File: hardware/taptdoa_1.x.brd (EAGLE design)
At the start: 64.8 x 63.2 mm, 60 parts, among them J1 105017-0001, U1 AP2112K-3.3TRG1, U2 STM32F103RBT6, Y1 8MHz

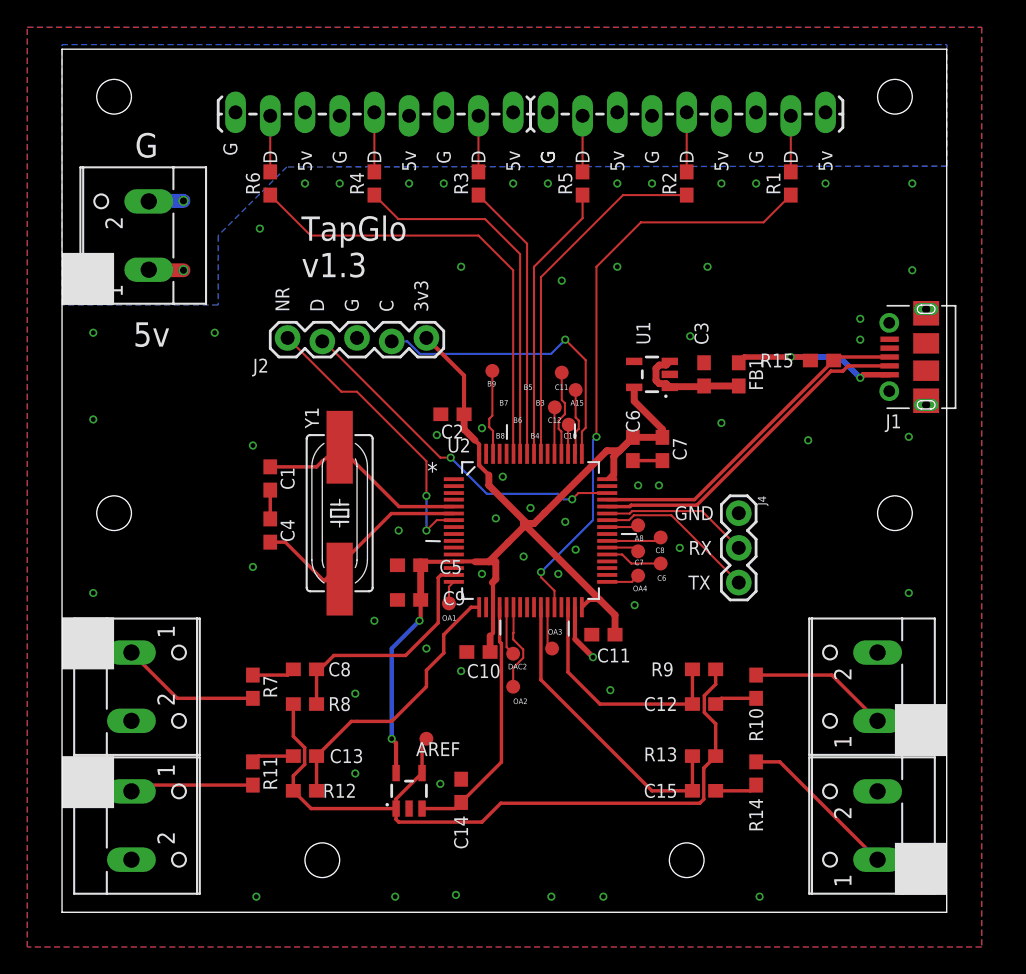
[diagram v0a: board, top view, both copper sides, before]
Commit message: re layout board
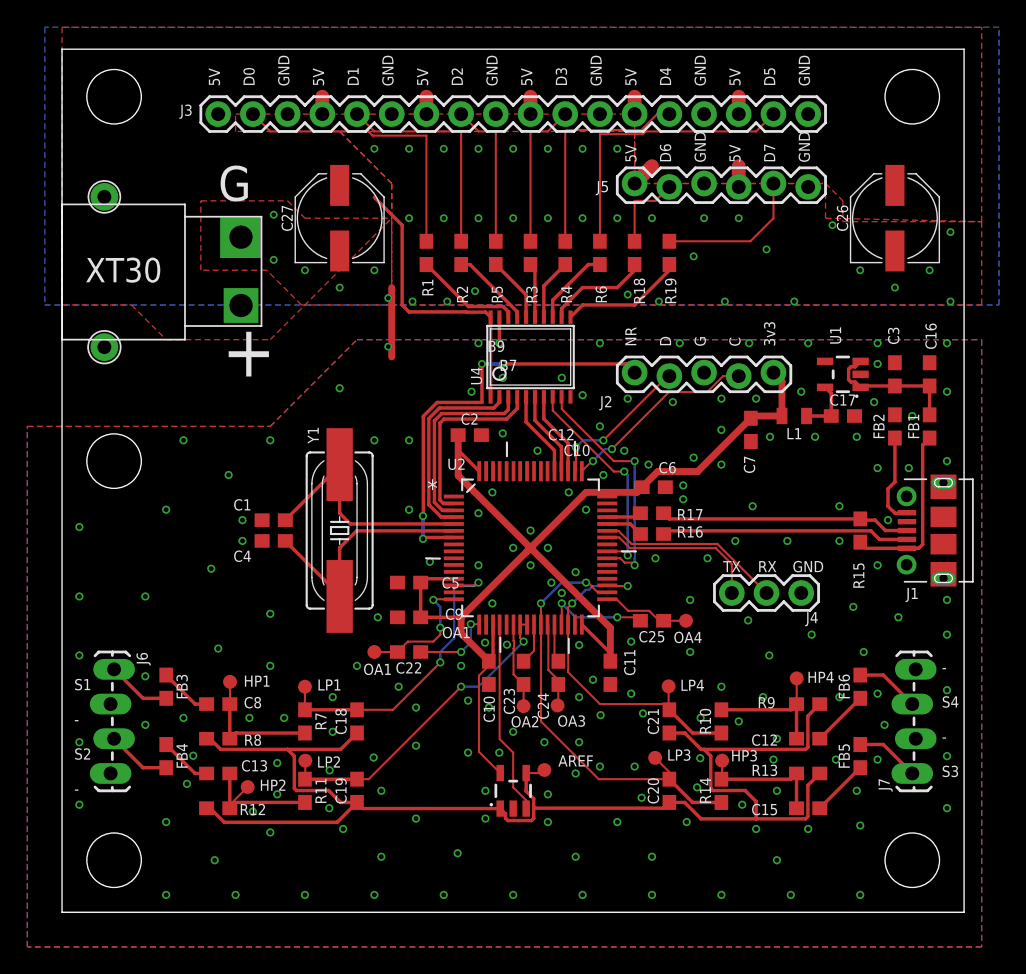
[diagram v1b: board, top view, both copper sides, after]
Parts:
- removed C14: 0.1uF, SparkFun-Capacitors:0603
- removed TP13, TP14, TP15, TP16, TP18, TP19, TP20: TEST-POINT3X4, SparkFun-Connectors:PAD.03X.04
- removed X1, X2, X3, X4, X5: (no value), con-wago-500:W237-102
- added C16: 0.1uF, SparkFun-Capacitors:0603
- added C17: 1.0uF, SparkFun-Capacitors:0603
- added C18, C19, C20, C21, C22, C23, C24, C25: 1nF, SparkFun-Capacitors:0603
- added C26, C27: 100uF, SparkFun-Capacitors:PANASONIC_D
- added FB2, FB3, FB4, FB5, FB6: 30Ω/1.8A, SparkFun-Coils:0603
- added J6, J7: (no value), SparkFun-Connectors:1X04_LOCK_LONGPADS
- added L1: 3.3µH/±20%/450mA, SparkFun-Coils:0805
- added R16, R17: 33, SparkFun-Resistors:0603
- added R18, R19: 75, SparkFun-Resistors:0603
- added TP3, TP4, TP5, TP6, TP7: TEST-POINT3X4, SparkFun-Connectors:PAD.03X.04
- added U$2: XT30XT30_THRUHOLE, XT30Male:ZT30
- added U4: SN74HCT245PWR, scanlime:TSSOP20
- C12, C13, C15, C8: value 100pF -> 1nF
- C3: value 1.0uF -> 4.7uF
- J3: device SparkFun-Connectors:1X09_LOCK_LONGPADS -> SparkFun-Connectors:1X18
- J5: device SparkFun-Connectors:1X09_LOCK_LONGPADS -> SparkFun-Connectors:1X06_LOCK
- R1, R2, R3, R4, R5, R6: value 100 -> 75
- R10, R11, R14, R7: value 1k -> 10k
- R12, R13, R8, R9: value 100k -> 10k
- moved TP10 35.4 mm to (13.6, 9.17)
- moved TP9 33.2 mm to (12.3, 16.9)
- moved J5 29.6 mm to (41.9, 53.3)
- moved TP11 29.2 mm to (48.3, 11.1)
- moved TP8 27.4 mm to (17.8, 16.5)
- moved R1 27.1 mm to (26.7, 48.3)
- moved J2 25.5 mm to (41.9, 39.4)
- moved TP1 24.9 mm to (36.3, 15.1)
- moved R6 24.7 mm to (39.4, 48.3)
- moved J3 24.1 mm to (11.4, 58.4)
- moved R2 17.3 mm to (29.2, 48.3)
- moved TP12 16.1 mm to (53.8, 17.1)
- moved R4 14.9 mm to (36.8, 48.3)
- moved FB1 14.5 mm to (63.5, 35.6), turned to 90 degrees
- moved C3 14.0 mm to (61.0, 39.4)
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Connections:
- removed net +5V: J3.3, J3.6, J3.9, J5.3, J5.6, J5.9, X1.1
- removed net DAC1_OUT2: TP19.P$1, U2.21
- removed net N$1: R7.2, X2.1
- removed net N$3: R11.2, X4.1
- removed net N$5: R14.2, X5.1
- removed net N$7: C12.2, R10.1
- removed net OPAMP1_IN: C13.1, R12.2, U2.17
- removed net OPAMP1_OUT: TP18.P$1, U2.16
- removed net OPAMP2_IN: C15.1, R13.2, U2.26
- removed net OPAMP2_OUT: TP20.P$1, U2.22
- removed net OPAMP3_IN: C8.1, R8.2, U2.15
- removed net OPAMP3_OUT: TP2.P$1, U2.27
- removed net OPAMP4_IN: C12.1, R9.2, U2.30
- removed net OPAMP4_OUT: TP14.P$1, U2.33
- removed net PA0-WKUP: U2.14
- removed net PA15: TP11.P$1, U2.50
- removed net PA7: U2.23
- removed net PA8: TP12.P$1, U2.41
- removed net PB10: U2.29
- removed net PB13: U2.34
- removed net PB14: U2.35
- removed net PB15: U2.36
- removed net PB2: R1.1, U2.28
- removed net PB3: R2.1, U2.55
- removed net PB4: R5.1, U2.56
- removed net PB5: R3.1, U2.57
- removed net PB6: R4.1, U2.58
- removed net PB7: R6.1, U2.59
- removed net PB8: U2.61
- removed net PB9: TP1.P$1, U2.62
- removed net PC10: TP10.P$1, U2.51
- removed net PC11: TP9.P$1, U2.52
- removed net PC12: TP8.P$1, U2.53
- removed net PC13-TAMPER-RTC: U2.2
- removed net PC14-OSC32_IN: U2.3
- removed net PC15-OSC32_OUT: U2.4
- removed net PC6: TP16.P$1, U2.37
- removed net PC7: TP13.P$1, U2.38
- removed net PC8: TP15.P$1, U2.39
- removed net PC9: U2.40
- removed net PD2: U2.54
- removed net VBAT: U2.1
- new net 5V: C26.+, C27.+, J3.1, J3.10, J3.13, J3.16, J3.4, J3.7, J5.1, J5.4, U$2.P$1, U4.1, U4.20
- new net HP1: C8.1, R7.2, R8.2, TP9.P$1
- new net HP2: C13.1, R11.2, R12.2, TP10.P$1
- new net HP3: C15.1, R13.2, R14.2, TP11.P$1
- new net HP4: C12.1, R10.2, R9.2, TP12.P$1
- new net N$10: R17.1, U2.45
- new net N$11: FB2.1, J1.5
- new net N$12: C17.1, L1.1, U1.5
- new net N$13: R1.1, U4.18
- new net N$14: R2.1, U4.17
- new net N$15: R5.1, U4.16
- new net N$16: R3.1, U4.15
- new net N$17: R4.1, U4.14
- new net N$18: R6.1, U4.13
- new net N$19: C8.2, FB3.1
- new net N$20: C15.2, FB5.1
- new net N$21: C13.2, FB4.1
- new net N$22: U2.53, U4.5
- new net N$23: C12.2, FB6.1
- new net N$24: U2.2, U4.4
- new net N$25: U2.3, U4.3
- new net N$26: U2.4, U4.2
- new net N$27: R18.1, U4.12
- new net N$28: R19.1, U4.11
- new net N$29: J5.2, R18.2
- new net N$30: J5.5, R19.2
- new net N$31: FB3.2, J6.1
- new net N$32: FB5.2, J7.1
- new net N$33: FB6.2, J7.3
- new net N$34: FB4.2, J6.3
- new net N$9: R16.1, U2.44
- new net OA1NEG: C22.1, U2.17
- new net OA1OUT: C22.2, TP4.P$1, U2.16
- new net OA2NEG: C23.1, U2.25
- new net OA2OUT: C23.2, TP3.P$1, U2.22
- new net OA3NEG: C24.1, U2.28
- new net OA3OUT: C24.2, TP1.P$1, U2.27
- new net OA4NEG: C25.2, U2.29
- new net OA4OUT: C25.1, TP2.P$1, U2.33
- new net SENSE1: C18.2, R7.1, TP8.P$1, U2.14, U2.15
- new net SENSE2: C19.2, R11.1, TP7.P$1, U2.23, U2.24
- new net SENSE3: C20.2, R14.1, TP6.P$1, U2.26, U2.34
- new net SENSE4: C21.2, R10.1, TP5.P$1, U2.30, U2.35
- net +3V3: now also L1.2; no longer U1.5
- net AREF: now also C18.1, C19.1, C20.1, C21.1
- net DAC1_OUT1: no longer C14.1
- net GND: now also C16.2, C17.2, C26.-, C27.-, FB2.2, J3.12, J3.15, J3.18, J3.3, J3.6, J3.9, J5.3, J5.6, J6.2, J6.4, J7.2, J7.4, U$2.P$2, U4.10, U4.19; no longer C14.2, J1.5, J3.1, J3.4, J3.7, J5.1, J5.4, J5.7, X1.2, X2.2, X3.2, X4.2, X5.2
- net LED0: now also J3.2; no longer J3.8
- net LED2: now also J3.8; no longer J3.2
- net LED3: now also J3.11; no longer J5.8
- net LED4: now also J3.14; no longer J5.5
- net LED5: now also J3.17; no longer J5.2
- net N$2: now also U2.39, U4.9; no longer C13.2, R11.1
- net N$4: now also U2.40, U4.8; no longer C15.2, R14.1
- net N$6: now also U2.51, U4.7; no longer R10.2, X3.1
- net N$8: now also U2.52, U4.6; no longer C8.2, R7.1
- net PA13: now also U2.50; no longer U2.46
- net USB_DM: now also R16.2; no longer U2.44
- net USB_DP: now also R17.2; no longer U2.45
- net VUSB2: now also C16.1
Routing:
- net PB2: track 43.4 -> 0.00 mm, vias 2 -> 0
- net AREF: track 55.8 -> 97.2 mm
- net PB7: track 33.5 -> 0.00 mm
- net SENSE3: track 0.00 -> 32.6 mm, vias 0 -> 2
- net 5V: track 0.00 -> 30.8 mm
- net PB6: track 27.1 -> 0.00 mm
- net SENSE4: track 0.00 -> 26.1 mm, vias 0 -> 2
- net PB3: track 26.1 -> 0.00 mm
- net SENSE2: track 0.00 -> 23.4 mm, vias 0 -> 2
- net SENSE1: track 0.00 -> 23.3 mm, vias 0 -> 2
- net OPAMP2_IN: track 22.3 -> 0.00 mm
- net OPAMP1_IN: track 20.4 -> 0.00 mm
- net PB4: track 20.4 -> 0.00 mm
- net PB5: track 20.4 -> 0.00 mm
- net OPAMP3_IN: track 17.5 -> 0.00 mm
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- added copper zone on layer 1, net 5V
- removed copper zone on layer 16, net +5V
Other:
- board size 64.8 x 63.2 mm -> 66 x 63.2 mm
- board text added: "-"
- board text added: "5V"
- board text added: "D0"
- board text added: "D1"
- board text added: "D2"
- board text added: "D3"
- board text added: "D4"
- board text added: "D5"
- board text added: "D6"
- board text added: "D7"
- board text added: "HP1"
- board text added: "HP2"
- board text added: "HP3"
- board text added: "HP4"
- board text added: "LP1"
- board text added: "LP2"
- board text added: "LP3"
- board text added: "LP4"
- board text added: "S1"
- board text added: "S2"
- board text added: "S3"
- board text added: "S4"
- board text removed: "5v"
- board text removed: "A15"
- board text removed: "A8"
- board text removed: "B3"
- board text removed: "B4"
- board text removed: "B5"
- board text removed: "B6"
- board text removed: "B8"
- board text removed: "C11"
- board text removed: "C6"
- board text removed: "C7"
- board text removed: "C8"
- board text removed: "DAC2"
- board text removed: "TapGlo v1.3"
